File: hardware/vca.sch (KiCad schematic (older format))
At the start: 59 parts

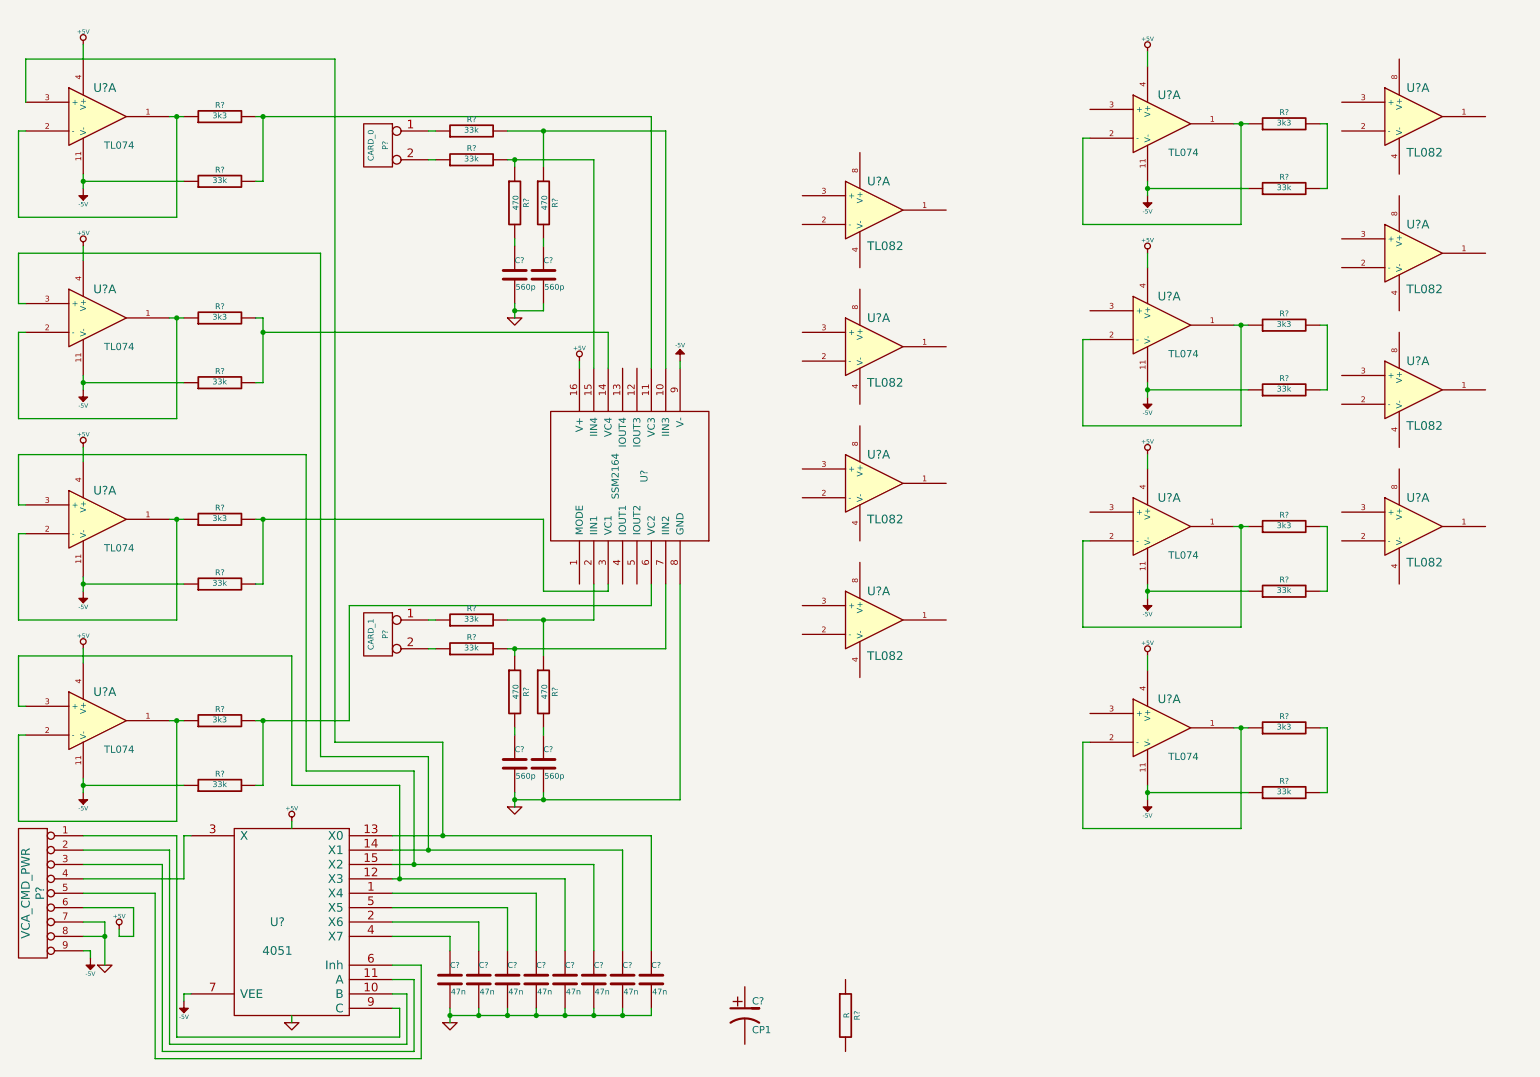
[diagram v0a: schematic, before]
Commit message: adding vca board schematics
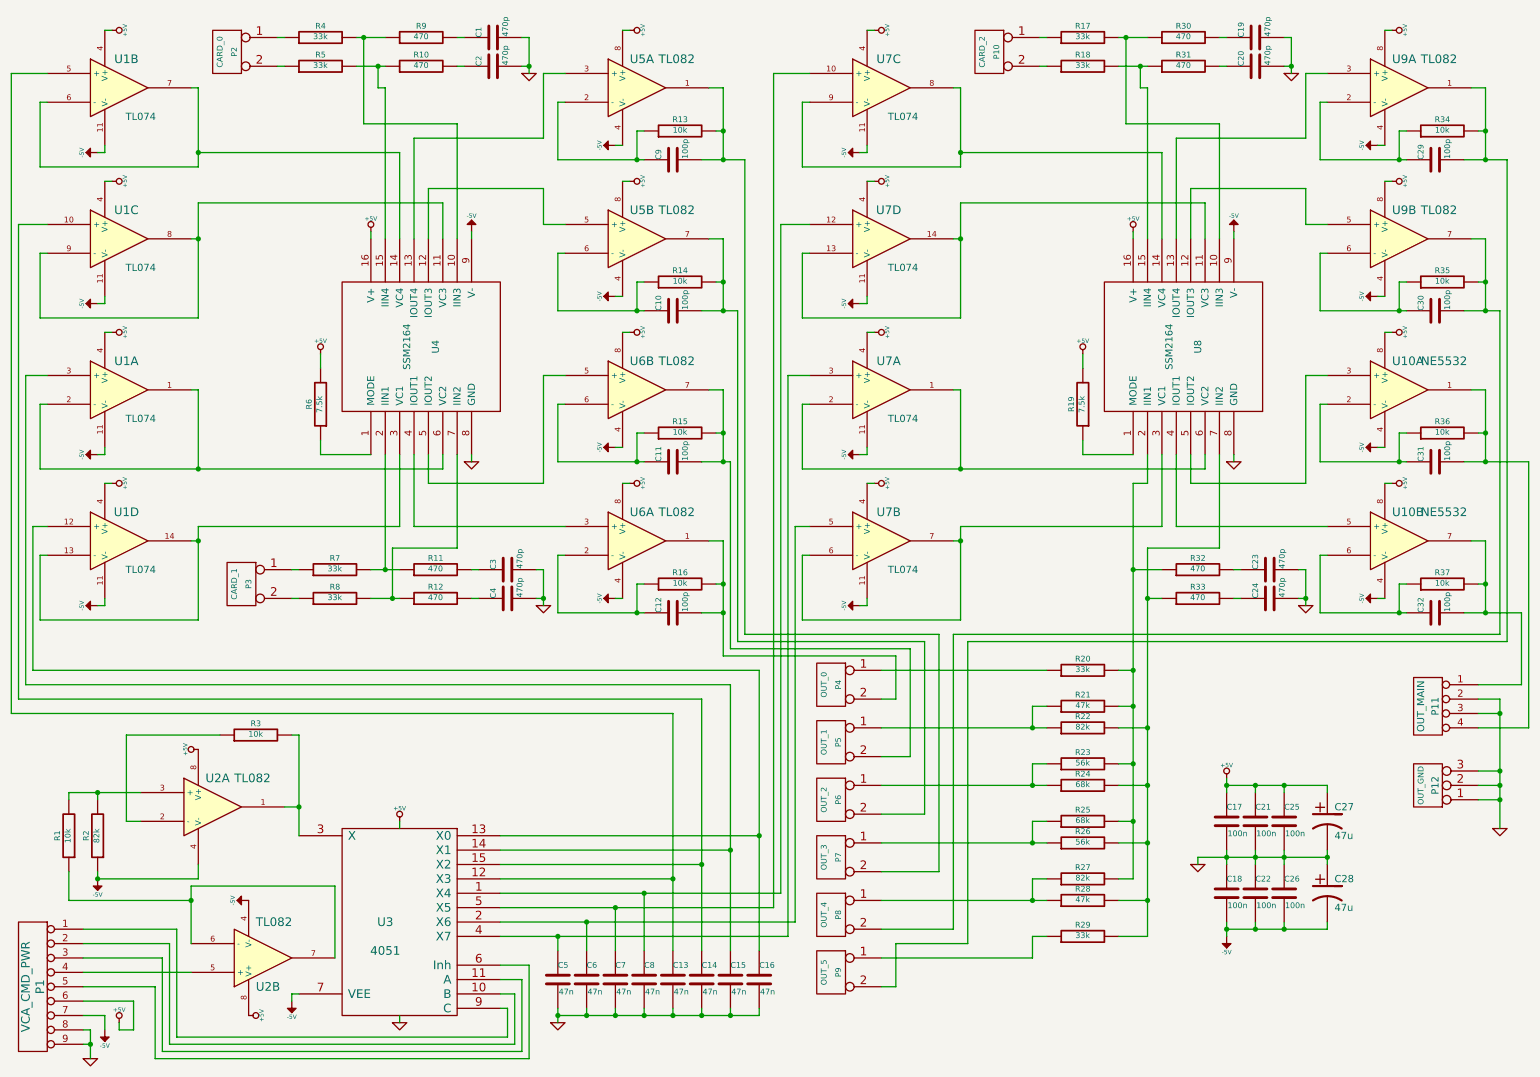
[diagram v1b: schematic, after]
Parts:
- removed C?: CP1, ~, symbol CP1
- removed C? (x2): 560p, ~, symbol C
- removed P?: CARD_0, symbol CONN_2
- removed R?: R, ~, symbol R
- removed R? (x10): 33k, ~, symbol R
- removed R? (x8): 3k3, ~, symbol R
- removed R? (x2): 470, ~, symbol R
- removed U? (x7): TL082, symbol TL082
- removed U? (x7): TL074, symbol TL074
- added C1, C19, C2, C20, C23, C24: 470p, ~, symbol C
- added C10, C11, C12, C29, C30, C31, C32, C9: 100p, ~, symbol C
- added C17, C18, C21, C22, C25, C26: 100n, ~, symbol C
- added C27, C28: 47u, ~, symbol CP1
- added P10: CARD_2, symbol CONN_2
- added P11: OUT_MAIN, symbol CONN_4
- added P12: OUT_GND, symbol CONN_3
- added P2: CARD_0, symbol CONN_2
- added P4: OUT_0, symbol CONN_2
- added P5: OUT_1, symbol CONN_2
- added P6: OUT_2, symbol CONN_2
- added P7: OUT_3, symbol CONN_2
- added P8: OUT_4, symbol CONN_2
- added P9: OUT_5, symbol CONN_2
- added R1, R13, R14, R15, R16, R3, R34, R35, R36, R37: 10k, ~, symbol R
- added R10, R30, R31, R32, R33, R9: 470, ~, symbol R
- added R17, R18, R20, R29, R4, R5: 33k, ~, symbol R
- added R19, R6: 7.5k, ~, symbol R
- added R2, R22, R27: 82k, ~, symbol R
- added R21, R28: 47k, ~, symbol R
- added R23, R26: 56k, ~, symbol R
- added R24, R25: 68k, ~, symbol R
- added unit 3 of U1
- added unit 1 of U1
- added unit 4 of U1
- added U10: NE5532, symbol TL082
- added U2, U6, U9: TL082, symbol TL082
- added unit 2 of U5
- added U7: TL074, symbol TL074
- added U8: SSM2164, MODULE, symbol SSM2164
- C3, C4: renamed from C?; value 560p -> 470p
- gave numbers to parts that had none: 18
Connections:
- net +5V: now also U5.8 (V+), C17.1, C21.1, C25.1, C27.1, R19.2, R6.2, U1.4 (V+), U1.4 (V+), U1.4 (V+), U10.8 (V+), U10.8 (V+), U2.8 (V+), U2.8 (V+), U5.8 (V+), U6.8 (V+), U6.8 (V+), U7.4 (V+), U7.4 (V+), U7.4 (V+), U7.4 (V+), U8.16 (V+), U9.8 (V+), U9.8 (V+)
- net -5V: now also P1.7 (P7), U5.4 (V-), C18.2, C22.2, C26.2, C28.2, R2.1, U1.11 (V-), U1.11 (V-), U1.11 (V-), U10.4 (V-), U10.4 (V-), U2.4 (V-), U2.4 (V-), U5.4 (V-), U6.4 (V-), U6.4 (V-), U7.11 (V-), U7.11 (V-), U7.11 (V-), U7.11 (V-), U8.9 (V-), U9.4 (V-), U9.4 (V-); no longer P1.9 (P9)
- net GND: now also P1.9 (P9), C1.2, C17.2, C18.1, C19.2, C2.2, C20.2, C21.2, C22.1, C23.2, C24.2, C25.2, C26.1, C27.2, C28.1, P11.2 (P2), P11.3 (P3), P12.1 (P1), P12.2 (PM), P12.3 (P3), U8.8 (GND); no longer P1.7 (P7)
- net at C8.1, U3.1 (X4): now also U7.12 (+)
- net at C13.1, U3.12 (X3): now also U1.5 (+)
- net at C16.1, U3.13 (X0): now also U1.12 (+); no longer U1.3 (+)
- net at C15.1, U3.14 (X1): now also U1.3 (+)
- net at C14.1, U3.15 (X2): now also U1.10 (+)
- net at C6.1, U3.2 (X6): now also U7.5 (+)
- net at U3.3 (X): now also R3.2, U2.1; no longer P1.4 (P4)
- net at C5.1, U3.4 (X7): now also U7.3 (+)
- net at C7.1, U3.5 (X5): now also U7.10 (+)
- net at U4.1 (MODE): now also R6.1
- net at U4.10 (IIN3): now also R4.2, R9.1
- net at U4.11 (VC3): now also U1.8, U1.9 (-)
- net at U4.12 (IOUT3): now also U5.5 (+)
- net at U4.13 (IOUT4): now also U5.3 (+)
- net at U4.14 (VC4): now also U1.6 (-), U1.7
- net at U4.15 (IIN4): now also R10.1, R5.2
- net at U4.3 (VC1): now also U1.13 (-), U1.14
- net at U4.4 (IOUT1): now also U6.3 (+)
- net at U4.5 (IOUT2): now also U6.5 (+)
- net at U4.6 (VC2): now also U1.1, U1.2 (-)
- net at U5.1: now also C9.2, P7.2 (PM), R13.2
- net at U5.2 (-): now also C9.1, R13.1
- new net: P1.4 (P4), U2.5 (+)
- new net: C10.1, R14.1, U5.6 (-)
- new net: C10.2, P6.2 (PM), R14.2, U5.7
- new net: C11.1, R15.1, U6.6 (-)
- new net: C11.2, P5.2 (PM), R15.2, U6.7
- new net: C12.2, P4.2 (PM), R16.2, U6.1
- new net: C12.1, R16.1, U6.2 (-)
- new net: P2.1 (P1), R4.1
- new net: P2.2 (PM), R5.1
- new net: C2.1, R10.2
- new net: C1.1, R9.2
- new net: P7.1 (P1), R25.1, R26.1
- new net: R22.2, R24.2, R26.2, R28.2, R29.2, R33.1, U8.7 (IIN2)
- new net: P8.1 (P1), R27.1, R28.1
- new net: R20.2, R21.2, R23.2, R25.2, R27.2, R32.1, U8.2 (IIN1)
- new net: P9.1 (P1), R29.1
- new net: P6.1 (P1), R23.1, R24.1
- new net: P5.1 (P1), R21.1, R22.1
- new net: P4.1 (P1), R20.1
- new net: R1.2, R2.2, U2.3 (+)
- new net: R1.1, U2.6 (-), U2.7
- new net: R19.1, U8.1 (MODE)
- new net: R3.1, U2.2 (-)
- new net: R17.2, R30.1, U8.10 (IIN3)
- new net: U7.13 (-), U7.14, U8.11 (VC3)
- new net: U8.12 (IOUT3), U9.5 (+)
- new net: U8.13 (IOUT4), U9.3 (+)
- new net: U7.8, U7.9 (-), U8.14 (VC4)
- new net: R18.2, R31.1, U8.15 (IIN4)
- new net: U7.6 (-), U7.7, U8.3 (VC1)
- new net: U10.5 (+), U8.4 (IOUT1)
- new net: U10.3 (+), U8.5 (IOUT2)
- new net: U7.1, U7.2 (-), U8.6 (VC2)
- new net: C29.2, P9.2 (PM), R34.2, U9.1
- new net: C29.1, R34.1, U9.2 (-)
- new net: C30.1, R35.1, U9.6 (-)
- new net: C30.2, P8.2 (PM), R35.2, U9.7
- new net: C31.2, P11.4 (P4), R36.2, U10.1
- new net: C31.1, R36.1, U10.2 (-)
- new net: C32.1, R37.1, U10.6 (-)
- new net: C32.2, P11.1 (P1), R37.2, U10.7
- new net: P10.1 (P1), R17.1
- new net: P10.2 (PM), R18.1
- new net: C20.1, R31.2
- new net: C19.1, R30.2
- new net: C24.1, R33.2
- new net: C23.1, R32.2
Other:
- moved on the sheet: C13, C14, C15, C16, C3, C4, C5, C6, C7, C8, P1, P3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
